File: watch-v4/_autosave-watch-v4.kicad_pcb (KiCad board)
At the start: 4 copper layers, 35 x 35 mm, 35 parts, among them J1 CONN_10, P1 array connection, Q1 MOSFET_P, SW1 SPST, SW2 SPST, SW3 SPST, U1 IC_MCP73831, U2 MAX1722, U3 DS3231, U4 LSM9DS0, U5 NRF51822, U6 BALUN, X1 16mhz

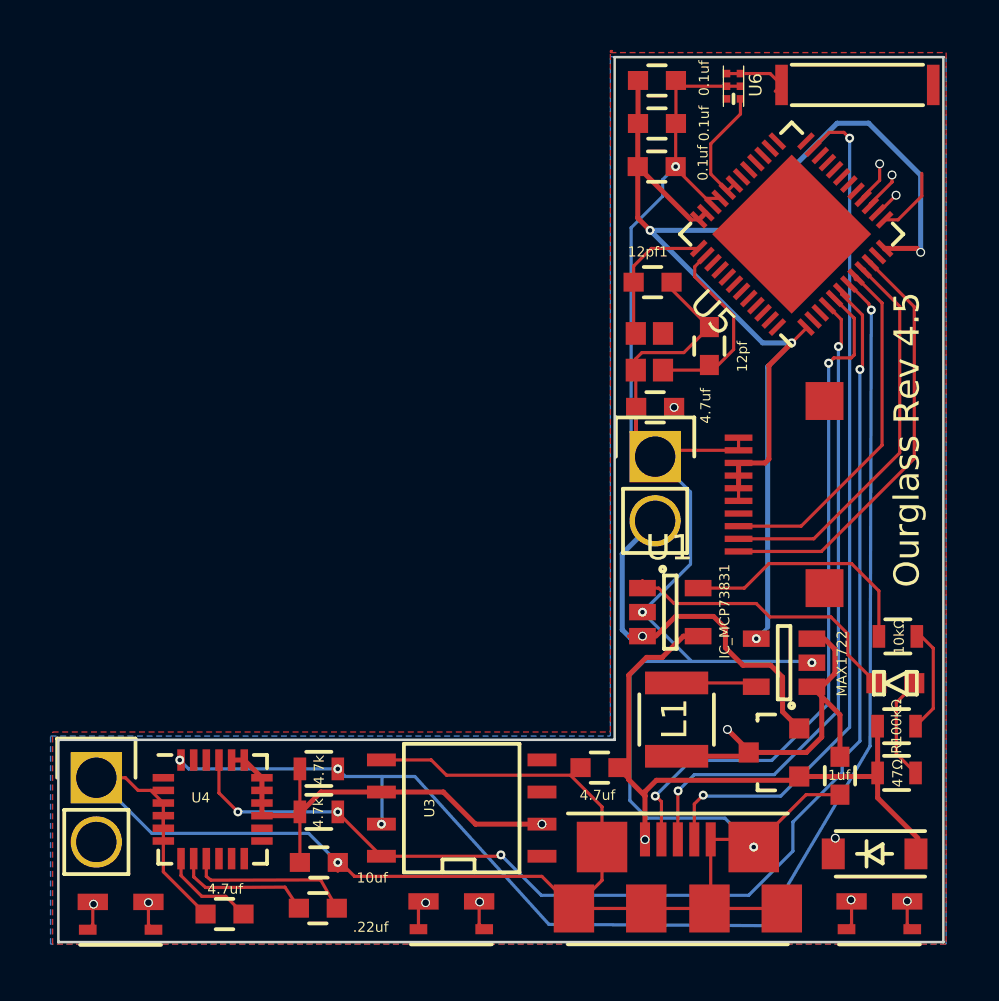
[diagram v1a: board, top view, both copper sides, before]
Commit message: up to version 5.2
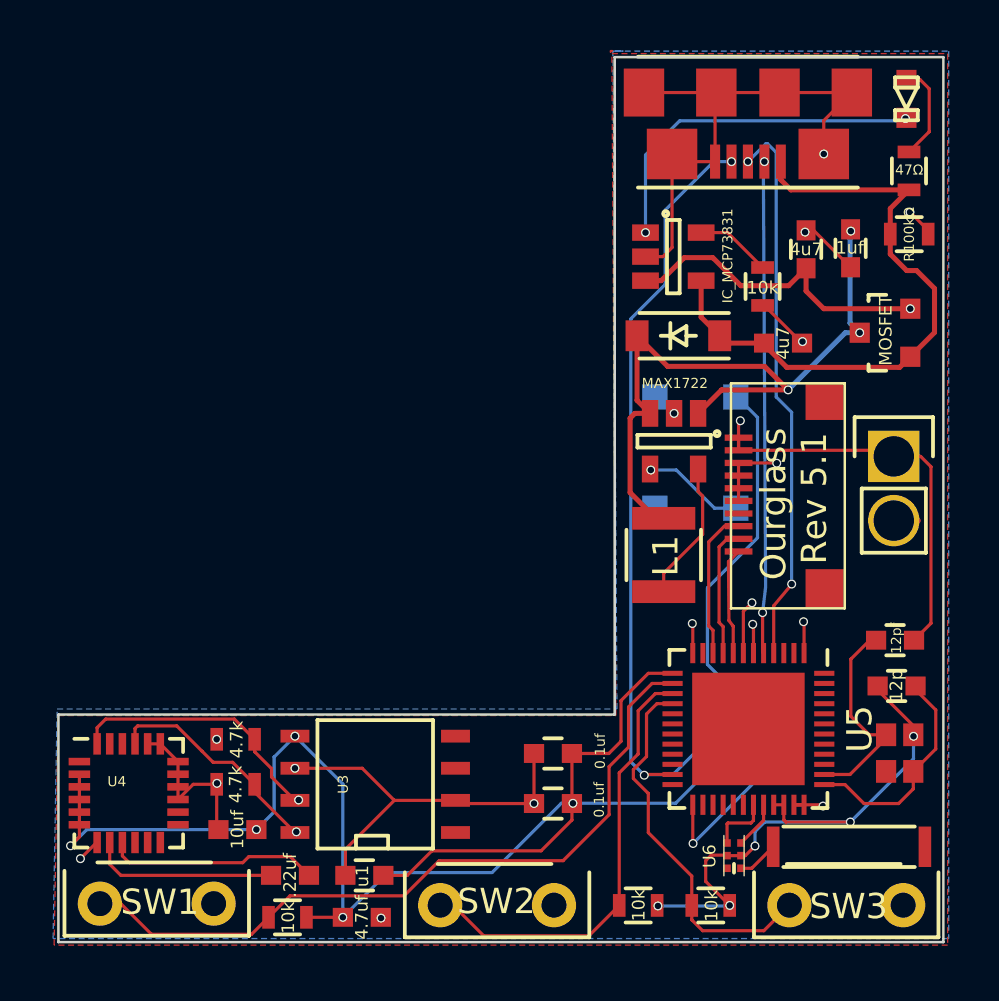
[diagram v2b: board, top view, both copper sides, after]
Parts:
- removed 12pf1: C9, Capacitors_SMD:C_0603
- removed P1: array connection, watch-v4:Pin_Header_Straight_1x02
- added 12p: C9, Capacitors_SMD:C_0603, F.Cu at (183.3, 105.6)
- added R4: 10k, Resistors_SMD:R_0603, F.Cu at (159.3, 114.7)
- added R7: 10k, Resistors_SMD:R_0603, F.Cu at (173.1, 114.2)
- added R8: 10k, Resistors_SMD:R_0603, F.Cu at (176.0, 114.2)
- added U7: NeoPixel, LEDs:Neopixel, B.Cu at (175.4, 96.3)
- C2, C3: value 4.7uf -> 4u7
- C8: value 0.1uf -> u1
- Q1: value MOSFET_P -> MOSFET
- R2: value 10kΩ -> 10k
- SW1, SW2, SW3: footprint watch-v4:panasonic-evpav-switch -> watch-v4:SW_Tactile_SPST_Angled_no_anchors
- moved C8 31.9 mm to (162.3, 113.1)
- moved SW3 31.0 mm to (183.6, 114.2), turned to 180 degrees
- moved U6 30.4 mm to (176.9, 112.2)
- moved ANT1 30.1 mm to (181.5, 111.9)
- moved XL1 30.1 mm to (177.5, 83.3), turned to 180 degrees
- moved C13 26.9 mm to (169.8, 108.2)
- moved SW1 26.3 mm to (156.3, 114.2), turned to 180 degrees
- moved C14 25.5 mm to (169.8, 110.2)
- moved R1 23.8 mm to (183.8, 85.2), turned to 270 degrees
- moved D2 23.1 mm to (183.7, 82.3), turned to 90 degrees
- moved D1 21.9 mm to (174.7, 91.7)
- moved X1 20.9 mm to (184.1, 109.1), turned to 90 degrees
- moved C1 20.9 mm to (181.5, 88.3)
- moved U5 19.6 mm to (177.5, 107.3), turned to 270 degrees
- moved R3 19.5 mm to (183.8, 87.7)
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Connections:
- net Net-(SW1-Pad2) renamed /SW1
- net Net-(SW2-Pad2) renamed /SW2
- net Net-(SW3-Pad2) renamed /SW3
- U5 pad 10: DISPLAY_SS -> DISPLAY_SCK
- U5 pad 25: Net-(U5-Pad25) -> /Backlight
- U5 pad 32: Net-(U5-Pad31) -> Net-(U5-Pad32)
- U5 pad 8: DISPLAY_SCK -> DISPLAY_SS
- U6 pad 1: Net-(U5-Pad31) -> Net-(ANT1-Pad1)
- U6 pad 3: Net-(ANT1-Pad1) -> Net-(U5-Pad32)
- U6 pad 4: Net-(ANT1-Pad1) -> Net-(U5-Pad31)
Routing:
- net VCC: track 133.9 -> 92.6 mm, vias 8 -> 9
- net /SW3: track 52.4 -> 15.0 mm, vias 2 -> 0
- net /EXTVCC: track 48.4 -> 25.0 mm, vias 1 -> 0
- net /Backlight: track 0.00 -> 22.1 mm, vias 0 -> 1
- net /SW2: track 39.3 -> 17.7 mm, vias 2 -> 0
- net SDA: track 54.8 -> 33.9 mm, vias 4 -> 2
- net SCL: track 50.1 -> 31.6 mm, vias 4 -> 2
- net GND: track 135.4 -> 148.3 mm, vias 5 -> 16
- net DISPLAY_SS: track 17.0 -> 4.24 mm
- net DISPLAY_MOSI: track 15.6 -> 5.17 mm
- net Net-(C6-Pad1): track 3.77 -> 13.8 mm, vias 0 -> 2
- net DISPLAY_SCK: track 14.2 -> 5.91 mm
- net /RX: track 27.4 -> 19.5 mm
- net Net-(R2-Pad1): track 9.80 -> 3.00 mm
- net /Regulator_In: track 22.5 -> 28.0 mm, vias 2 -> 3
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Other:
- outline, holes or cut-outs redrawn
- board text added: "Ourglass Rev 5.1"
- board text removed: "Ourglass Rev 4.5"
